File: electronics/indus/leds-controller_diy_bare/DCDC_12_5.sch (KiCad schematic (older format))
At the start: 8 parts, among them U5 TL2575HV-12, U6 KA7805ERTF

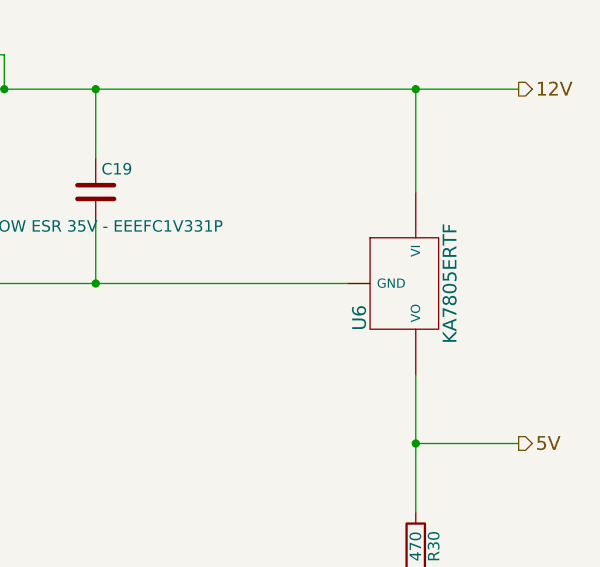
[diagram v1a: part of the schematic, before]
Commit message: before routing - no more errors
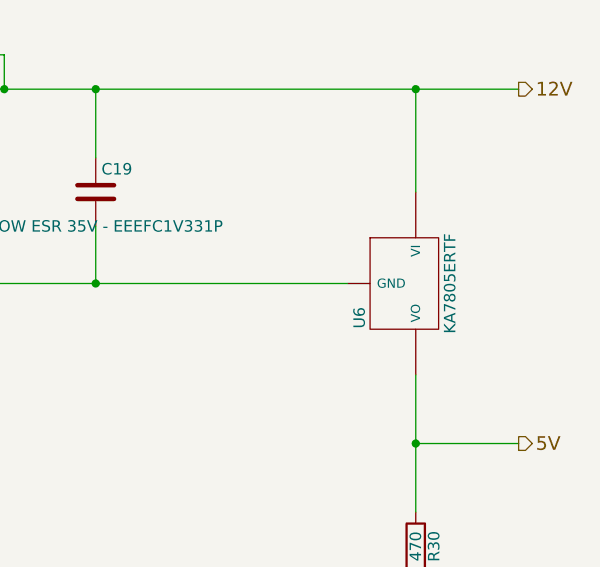
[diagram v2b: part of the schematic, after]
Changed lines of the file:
@@
 LIBS:contrib
 LIBS:valves
+LIBS:tps54335a
 LIBS:risebox
-LIBS:tps54335a
 LIBS:leds-controller-cache
 EELAYER 25 0
@@
 	3050 2950 4850 2950
 $Comp
-L GND #PWR018
+L GND #PWR017
 U 1 1 576240CC
 P 5650 4200
-F 0 "#PWR018" H 5650 3950 50  0001 C CNN
+F 0 "#PWR017" H 5650 3950 50  0001 C CNN
 F 1 "GND" H 5650 4050 50  0000 C CNN
 F 2 "" H 5650 4200 50  0000 C CNN
@@
 	8050 3950 8050 3700
 Connection ~ 6450 3950
-$Comp
-L 7805 U6
-U 1 1 576245A9
-P 9400 3950
-F 0 "U6" H 9550 3754 60  0000 C CNN
-F 1 "KA7805ERTF" H 9400 4150 60  0000 C CNN
-F 2 "risebox:KA7805ERTF_TO-252-3" H 9400 3950 60  0001 C CNN
-F 3 "" H 9400 3950 60  0000 C CNN
-	1    9400 3950
-	0    1    1    0
-$EndComp
 Wire Wire Line
 	9450 4350 9450 4950
@@
 	9450 5250 9450 5350
 $Comp
-L GND #PWR019
+L GND #PWR018
 U 1 1 5764C97D
 P 9450 6000
-F 0 "#PWR019" H 9450 5750 50  0001 C CNN
+F 0 "#PWR018" H 9450 5750 50  0001 C CNN
 F 1 "GND" H 9450 5850 50  0000 C CNN
 F 2 "" H 9450 6000 50  0000 C CNN
@@
 Wire Wire Line
 	5250 3550 5250 3950
+$Comp
+L 7805 U6
+U 1 1 576F3794
+P 9400 3950
+F 0 "U6" H 9550 3754 50  0000 C CNN
+F 1 "KA7805ERTF" H 9400 4150 50  0000 C CNN
+F 2 "risebox:KA7805ERTF_TO-252-3" H 9400 3950 50  0001 C CNN
+F 3 "" H 9400 3950 50  0000 C CNN
+	1    9400 3950
+	0    1    1    0
+$EndComp
 $EndSCHEMATC
